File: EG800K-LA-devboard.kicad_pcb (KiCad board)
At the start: 4 copper layers, 35 x 36.5 mm, 39 parts, among them J1 U.FL-R-SMT_10_, J2 MICROQTJ, J5 Conn_01x08_Pin, Q1 DTC143ZUAT106, Q2 DTC143ZUAT106, Q4 DTC143ZUAT106, Q5 DTC143ZUAT106, U4 EG800KEULC-I03-SNNSA

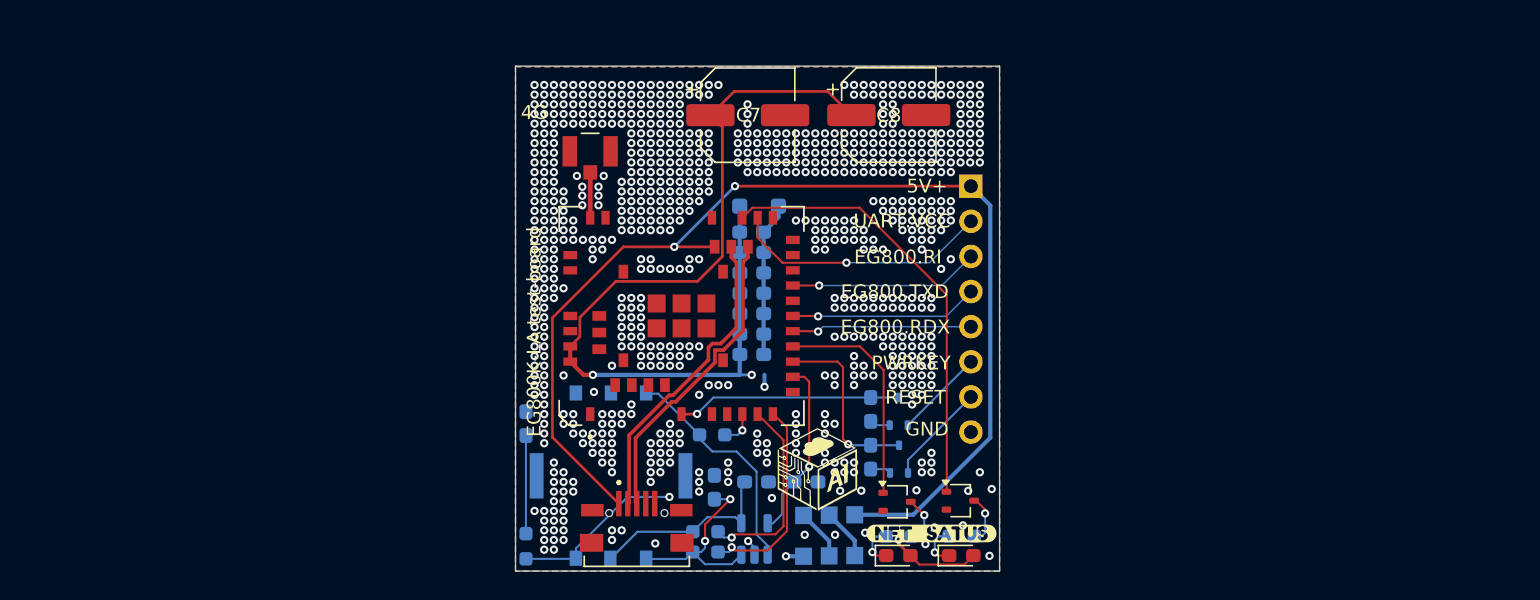
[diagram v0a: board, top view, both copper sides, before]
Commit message: cambios minimos
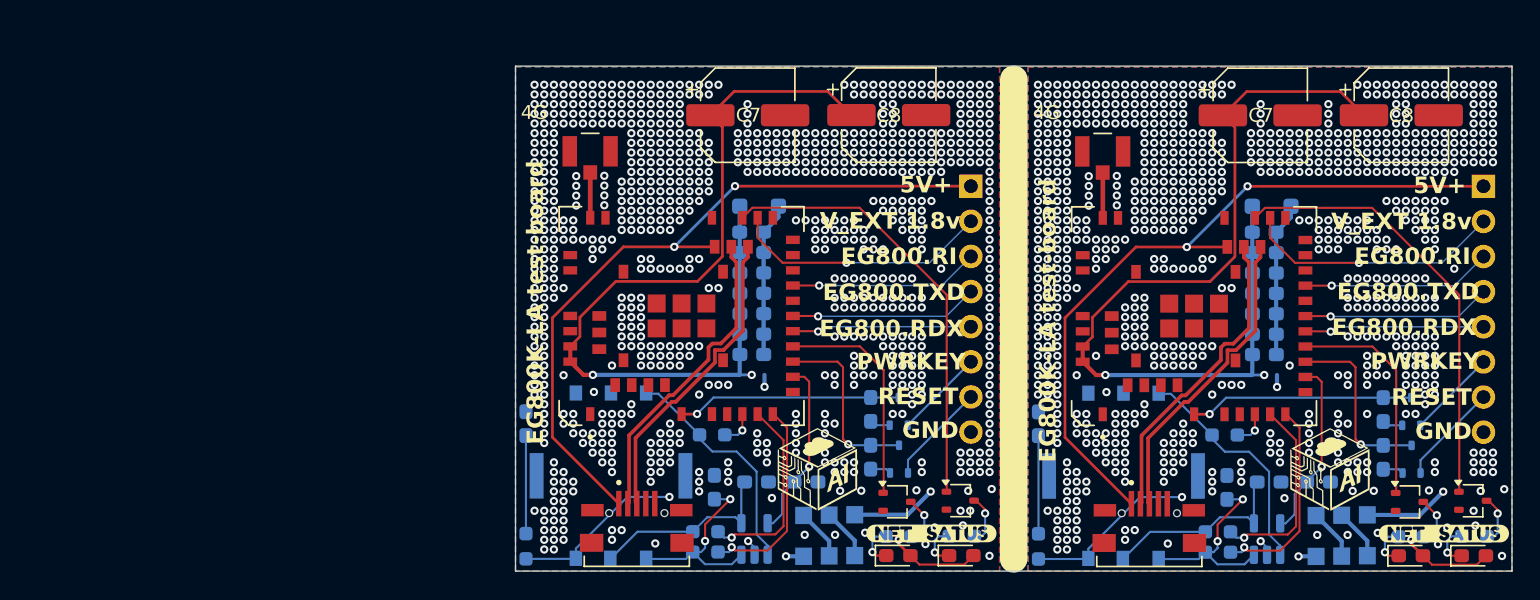
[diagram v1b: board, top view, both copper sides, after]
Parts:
- added C1: 33pF, Capacitor_SMD:C_0603_1608Metric_Pad1.08x0.95mm_HandSolder, B.Cu at (181.9, 85.2)
- added C2: 33pF, Capacitor_SMD:C_0603_1608Metric_Pad1.08x0.95mm_HandSolder, B.Cu at (195.6, 89.8)
- added C21: 47uf, Capacitor_SMD:C_0603_1608Metric_Pad1.08x0.95mm_HandSolder, B.Cu at (198.3, 80.2)
- added C22: 33pf, Capacitor_SMD:C_0603_1608Metric_Pad1.08x0.95mm_HandSolder, B.Cu at (198.3, 71.3)
- added C23: 100nf, Capacitor_SMD:C_0603_1608Metric_Pad1.08x0.95mm_HandSolder, B.Cu at (198.3, 72.8)
- added C24: 10nf, Capacitor_SMD:C_0603_1608Metric_Pad1.08x0.95mm_HandSolder, B.Cu at (198.3, 74.3)
- added C25: 0.1uf, Capacitor_SMD:C_0603_1608Metric_Pad1.08x0.95mm_HandSolder, B.Cu at (198.3, 75.7)
- added C26: 1uf, Capacitor_SMD:C_0603_1608Metric_Pad1.08x0.95mm_HandSolder, B.Cu at (198.3, 77.2)
- added C27: 10uf, Capacitor_SMD:C_0603_1608Metric_Pad1.08x0.95mm_HandSolder, B.Cu at (198.3, 78.7)
- added C3: 10nf, Capacitor_SMD:C_0603_1608Metric_Pad1.08x0.95mm_HandSolder, B.Cu at (206.9, 84.1)
- added C4: 33pF, Capacitor_SMD:C_0603_1608Metric_Pad1.08x0.95mm_HandSolder, B.Cu at (198.6, 89.4)
- added C5: 100nf, Capacitor_SMD:C_0603_1608Metric_Pad1.08x0.95mm_HandSolder, B.Cu at (202.2, 89.4)
- added C6: 10nf, Capacitor_SMD:C_0603_1608Metric_Pad1.08x0.95mm_HandSolder, B.Cu at (206.9, 87.6)
- added C7: 470uF, Capacitor_SMD:CP_Elec_6.3x7.7, F.Cu at (198.0, 62.9)
- added C8: 470uF, Capacitor_SMD:CP_Elec_6.3x7.7, F.Cu at (208.2, 62.9)
- added D1: ESDA6V1SC5, Package_TO_SOT_SMD:SOT-23-5, B.Cu at (198.5, 93.5)
- added D3: KUU SS36, Snapeda:KUU_SS36_foot, B.Cu at (205.7, 93.2)
- added D4: KUU SS36, Snapeda:KUU_SS36_foot, B.Cu at (203.9, 93.3)
- added D5: SMFJ5.0A, Diode_SMD:D_SOD-123F, B.Cu at (198.8, 69.4)
- added D6: LED, LED_SMD:LED_0603_1608Metric_Pad1.05x0.95mm_HandSolder, F.Cu at (213.4, 94.7)
- added D7: LED, LED_SMD:LED_0603_1608Metric_Pad1.05x0.95mm_HandSolder, F.Cu at (208.9, 94.7)
- added D8: KUU SS36, Snapeda:KUU_SS36_foot, B.Cu at (202.0, 93.3)
- added G***: LOGO, Images:LOGOv3.4, F.Cu at (203.0, 88.6)
- added J1: U.FL-R-SMT_10_, Snapeda:U.FL-R-SMT_10_-foot, F.Cu at (186.6, 65.5)
- added J2: MICROQTJ, Snapeda:MICROQTJ-foot, F.Cu at (189.9, 91.6)
- added J5: Conn_01x08_Pin, Connector_PinHeader_2.54mm:PinHeader_1x08_P2.54mm_Vertical, B.Cu at (214.1, 68.0)
- added NANO-SIM-0501A-P1: NANO-SIM-0501A-P, Snapeda:nano-sim-0501a-p_foot, B.Cu at (188.1, 88.9)
- added Q1: DTC143ZUAT106, Package_TO_SOT_SMD:SOT-323_SC-70, B.Cu at (208.9, 84.3)
- added Q2: DTC143ZUAT106, Package_TO_SOT_SMD:SOT-323_SC-70, B.Cu at (208.9, 87.7)
- added Q4: DTC143ZUAT106, Package_TO_SOT_SMD:SOT-323_SC-70, F.Cu at (213.3, 90.7)
- added Q5: DTC143ZUAT106, Package_TO_SOT_SMD:SOT-323_SC-70, F.Cu at (208.8, 90.8)
- added R1: 0, Resistor_SMD:R_0603_1608Metric_Pad0.98x0.95mm_HandSolder, B.Cu at (194.9, 93.0)
- added R16: 2.2k, Resistor_SMD:R_0603_1608Metric_Pad0.98x0.95mm_HandSolder, B.Cu at (213.4, 93.3)
- added R17: 2.2k, Resistor_SMD:R_0603_1608Metric_Pad0.98x0.95mm_HandSolder, B.Cu at (208.9, 93.3)
- added R2: 0, Resistor_SMD:R_0603_1608Metric_Pad0.98x0.95mm_HandSolder, B.Cu at (194.9, 94.5)
- added R3: 0, Resistor_SMD:R_0603_1608Metric_Pad0.98x0.95mm_HandSolder, B.Cu at (195.4, 86.0)
- added R4: 15k, Resistor_SMD:R_0603_1608Metric_Pad0.98x0.95mm_HandSolder, B.Cu at (181.9, 94.0)
- added U4: EG800KEULC-I03-SNNSA, Snapeda:Quectel_EG800K_foot_recorted, F.Cu at (193.2, 77.4)
- added kibuzzard-69C732A2: G***, kibuzzard-69C732A2, F.Cu at (211.2, 93.1)
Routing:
- net /DC 3.8v supply: track 127.5 -> 255.1 mm, vias 5 -> 10
- net +5V: track 83.4 -> 164.1 mm, vias 2 -> 6
- net /SIM_VDD: track 37.2 -> 74.5 mm, vias 2 -> 4
- net /EG800K.STATUS: track 31.9 -> 63.9 mm
- net /EG800K.USB_D+: track 22.5 -> 45.0 mm
- net /EG800K.USB_D-: track 22.5 -> 45.0 mm
- net /EG800K.VDD_ETX: track 18.9 -> 37.7 mm, vias 1 -> 2
- net Net-(NANO-SIM-0501A-P1-I/O): track 16.8 -> 33.6 mm
- net /EG800K.PWRKEY: track 16.2 -> 32.4 mm, vias 1 -> 2
- net /EG800K.NET_STATUS: track 16.2 -> 32.3 mm
- net GND: track 15.4 -> 30.7 mm, vias 767 -> 1612
- net /SIM_CLK: track 14.8 -> 29.6 mm, vias 1 -> 2
- net Net-(NANO-SIM-0501A-P1-CLK): track 14.2 -> 28.4 mm, vias 2 -> 4
- net /EG800K.UART1_TXD: track 14.1 -> 28.3 mm, vias 1 -> 2
- net /SIM_RST: track 14.1 -> 28.3 mm, vias 1 -> 2
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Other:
- board size 35 x 36.5 mm -> 72 x 36.5 mm
- board text added: "V_EXT 1.8v"
- board text added: "no tapered RF 0.3424 clear 0.5080 Coplanar Single Ended"
- board text added: "tapered RF 0.3424 clear 0.5080 Coplanar Single Ended"
- board text removed: "UART.VCC"

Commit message: original rediseñado
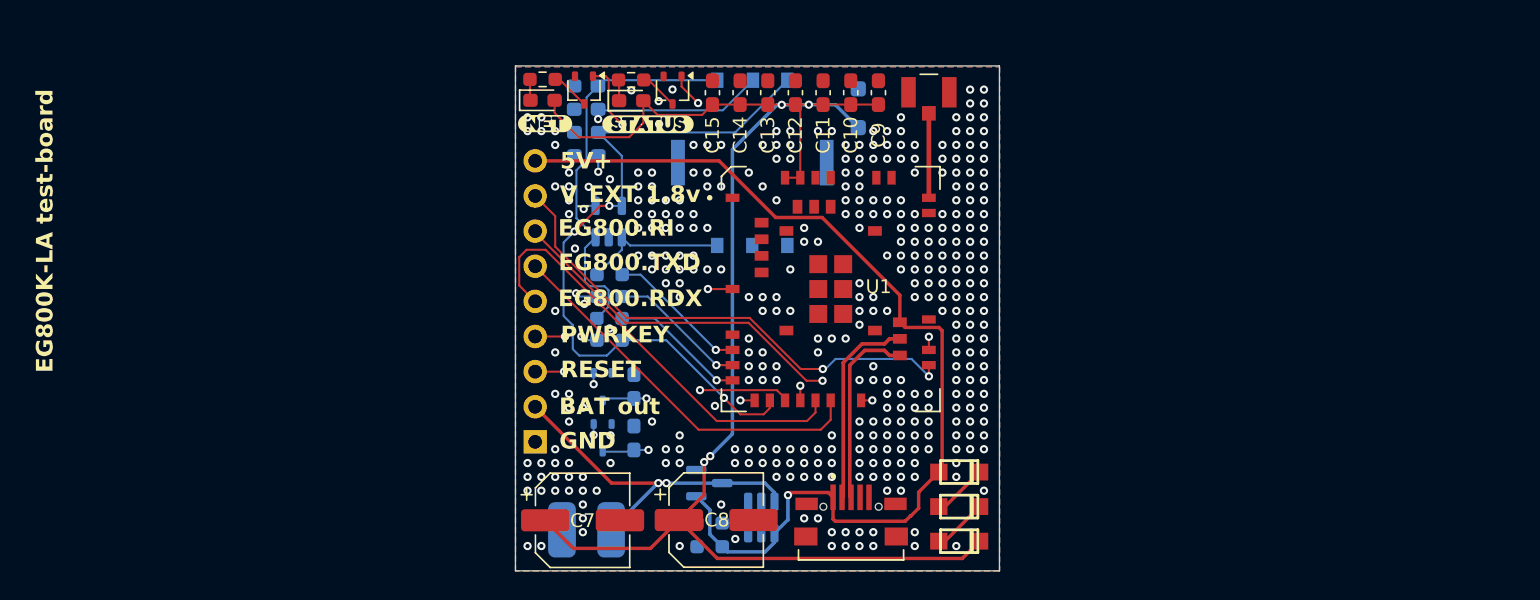
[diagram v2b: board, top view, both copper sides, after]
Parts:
- removed the C1 at (181.9, 85.2)
- removed the C2 at (195.6, 89.8)
- removed C21: 47uf, Capacitor_SMD:C_0603_1608Metric_Pad1.08x0.95mm_HandSolder
- removed C22: 33pf, Capacitor_SMD:C_0603_1608Metric_Pad1.08x0.95mm_HandSolder
- removed C23: 100nf, Capacitor_SMD:C_0603_1608Metric_Pad1.08x0.95mm_HandSolder
- removed C24: 10nf, Capacitor_SMD:C_0603_1608Metric_Pad1.08x0.95mm_HandSolder
- removed C25: 0.1uf, Capacitor_SMD:C_0603_1608Metric_Pad1.08x0.95mm_HandSolder
- removed C26: 1uf, Capacitor_SMD:C_0603_1608Metric_Pad1.08x0.95mm_HandSolder
- removed C27: 10uf, Capacitor_SMD:C_0603_1608Metric_Pad1.08x0.95mm_HandSolder
- removed the C3 at (206.9, 84.1)
- removed the C4 at (198.6, 89.4)
- removed the C5 at (202.2, 89.4)
- removed the C6 at (206.9, 87.6)
- removed the C7 at (198.0, 62.9)
- removed the C8 at (208.2, 62.9)
- removed the D1 at (198.5, 93.5)
- removed the D3 at (205.7, 93.2)
- removed the D4 at (203.9, 93.3)
- removed the D5 at (198.8, 69.4)
- removed the D6 at (213.4, 94.7)
- removed the D7 at (208.9, 94.7)
- removed D8: KUU SS36, Snapeda:KUU_SS36_foot
- removed G*** (x2): LOGO, Images:LOGOv3.4
- removed the J1 at (186.6, 65.5)
- removed the J2 at (189.9, 91.6)
- removed J5 (x2): Conn_01x08_Pin, Connector_PinHeader_2.54mm:PinHeader_1x08_P2.54mm_Vertical
- removed the NANO-SIM-0501A-P1 at (188.1, 88.9)
- removed the Q1 at (208.9, 84.3)
- removed the Q2 at (208.9, 87.7)
- removed the Q4 at (213.3, 90.7)
- removed the Q5 at (208.8, 90.8)
- removed the R1 at (194.9, 93.0)
- removed R16, R17: 2.2k, Resistor_SMD:R_0603_1608Metric_Pad0.98x0.95mm_HandSolder
- removed the R2 at (194.9, 94.5)
- removed the R3 at (195.4, 86.0)
- removed the R4 at (181.9, 94.0)
- removed U4 (x2): EG800KEULC-I03-SNNSA, Snapeda:Quectel_EG800K_foot_recorted
- removed kibuzzard-69C732A2 (x2): G***, kibuzzard-69C732A2
- added BAT+1: BAT+, Connector_Wire:SolderWirePad_1x01_SMD_2x4mm, B.Cu at (151.0, 92.8)
- added BAT-1: BAT-, Connector_Wire:SolderWirePad_1x01_SMD_2x4mm, B.Cu at (147.5, 92.8)
- added J3: Conn_01x09_Pin, Connector_PinHeader_2.54mm:PinHeader_1x09_P2.54mm_Vertical, B.Cu at (145.5, 86.5)
- added Q3: AO3415, Package_TO_SOT_SMD:SOT-23, B.Cu at (158.1, 89.5)
- added R5: 2.4K, Resistor_SMD:R_0603_1608Metric_Pad0.98x0.95mm_HandSolder, B.Cu at (158.2, 92.3)
- added R6: 10k, Resistor_SMD:R_0603_1608Metric_Pad0.98x0.95mm_HandSolder, B.Cu at (158.2, 94.1)
- added U1: EG800KEULC-I03-SNNSA, Snapeda:Quectel_EG800K_foot_recorted, F.Cu at (166.9, 75.4)
- added U2: TP4057, Package_TO_SOT_SMD:TSOT-23-6, B.Cu at (161.9, 92.0)
- added kibuzzard-6A166AE0: G***, kibuzzard-6A166AE0, F.Cu at (146.3, 63.5)
- added kibuzzard-6A166AEF: G***, kibuzzard-6A166AEF, F.Cu at (153.7, 63.5)
- C10: renamed from C22; moved to F.Cu
- C11: renamed from C23; moved to F.Cu
- C12: renamed from C24; moved to F.Cu
- C13: renamed from C25; moved to F.Cu
- C14: renamed from C26; moved to F.Cu
- C15: renamed from C27; moved to F.Cu
- C9: renamed from C21; moved to F.Cu
- D2: renamed from D3; moved to F.Cu
- D3: renamed from D4; moved to F.Cu
- D4: renamed from D8; moved to F.Cu
- R7: renamed from R16; moved to F.Cu
- R8: renamed from R17; moved to F.Cu
- moved R8 41.9 mm to (146.1, 60.3)
- moved D7 41.8 mm to (146.1, 61.8)
- moved R7 40.7 mm to (152.5, 60.3)
- moved D6 40.6 mm to (152.5, 61.8)
- moved Q5 37.4 mm to (149.1, 61.0), turned to -90 degrees
- moved C7 36.7 mm to (149.0, 92.2)
- moved Q4 36.2 mm to (155.5, 61.0), turned to -90 degrees
- moved C2 30.5 mm to (149.2, 60.8), turned to 0 degrees
- moved C4 29.9 mm to (149.2, 64.1), turned to 0 degrees
- moved C3 29.6 mm to (149.2, 62.4), turned to 0 degrees
- moved C8 29.4 mm to (158.6, 92.1)
- moved D1 25.3 mm to (150.9, 70.6)
- moved J1 24.9 mm to (174.0, 61.2)
- moved NANO-SIM-0501A-P1 24.8 mm to (161.2, 66.3), turned to 0 degrees
- moved Q2 21.5 mm to (150.4, 86.2), turned to -90 degrees
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- renumbered C4 to C3, C5 to C4, C3 to C5, C8 to C7, C7 to C8
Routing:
- net /DC 3.8v supply: track 255.1 -> 108.7 mm, vias 10 -> 4
- net +5V: track 164.1 -> 73.4 mm, vias 6 -> 1
- net /EG800K.STATUS: track 63.9 -> 27.2 mm, vias 0 -> 2
- net /EG800K.USB_D+: track 45.0 -> 13.9 mm
- net /EG800K.USB_D-: track 45.0 -> 14.7 mm
- net GND: track 30.7 -> 1.03 mm, vias 1612 -> 363
- net +4.2V: track 0.00 -> 25.9 mm, vias 0 -> 2
- net Net-(NANO-SIM-0501A-P1-I/O): track 33.6 -> 10.6 mm
- net /SIM_VDD: track 74.5 -> 52.4 mm, vias 4 -> 3
- net /SIM_CLK: track 29.6 -> 9.84 mm, vias 2 -> 1
- net /SIM_RST: track 28.3 -> 10.0 mm, vias 2 -> 1
- net /EG800K.PWRKEY: track 32.4 -> 14.8 mm
- net /EG800K.RESET: track 26.5 -> 15.8 mm
- net /HOST.EG800K.RESET: track 14.8 -> 8.35 mm, vias 0 -> 2
- net /HOST.EG800K.PWRKEY: track 13.0 -> 7.35 mm, vias 0 -> 2
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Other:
- board size 72 x 36.5 mm -> 35 x 36.5 mm
- board text added: "BAT out"
- board text removed: "10K.FET.10K"
- board text removed: "4G"
- board text removed: "Luis D."
- board text removed: "R0"
- board text removed: "no tapered RF 0.3424 clear 0.5080 Coplanar Single Ended"
